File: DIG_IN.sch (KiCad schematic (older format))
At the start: 12 parts, among them U8 PC817

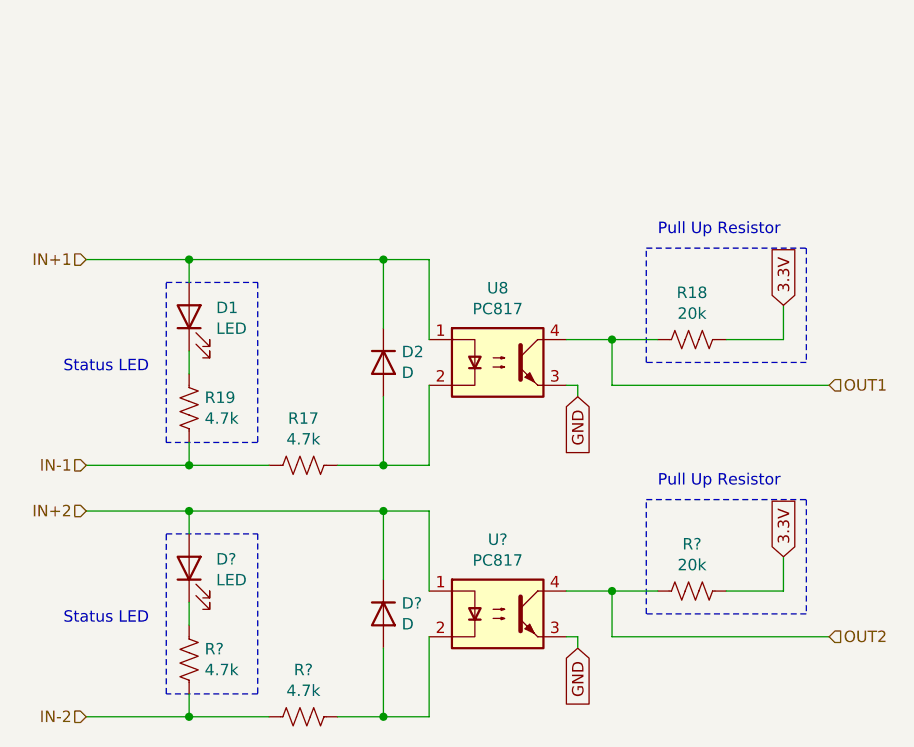
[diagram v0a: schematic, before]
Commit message: Testing and adjustments
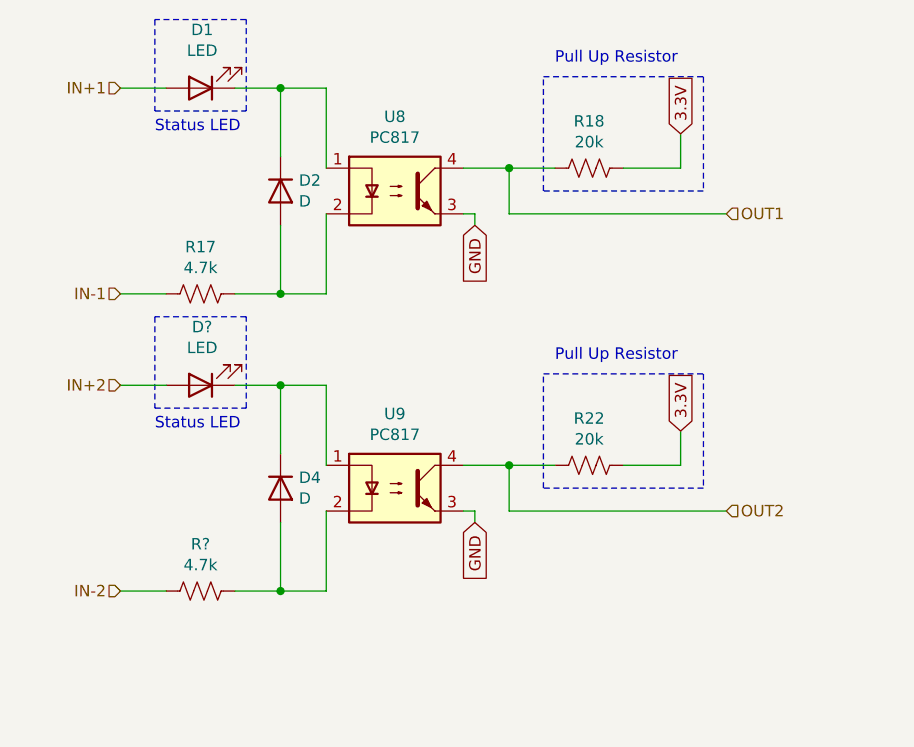
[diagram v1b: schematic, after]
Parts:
- removed D?: LED, symbol Device:LED
- removed R19, R? (x2): 4.7k, symbol Device:R_US
- added D?: LED, symbol Device:LED
- added R?: 4.7k, symbol Device:R_US
- gave numbers to parts that had none: 3
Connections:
- net IN+1: no longer D2.1 (K), U8.1
- net IN+2: now also D?.2 (A); no longer D4.1 (K), U9.1
- net IN-2: now also R?.2
- net at D1.1 (K): now also D2.1 (K), U8.1
- net at D4.2 (A), U9.2: now also R?.1
- new net: D4.1 (K), D?.1 (K), U9.1
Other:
- moved on the sheet: D1, D2, D4, R17, R18, R22, U8, U9
